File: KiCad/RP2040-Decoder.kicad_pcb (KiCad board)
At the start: 2 copper layers, 25 x 20 mm, 57 parts, among them J1 T0, J10 2, J11 3, J12 4, J13 5, J14 +V, J15 M_OUT_B, J16 M_OUT_A, J17 GND, J18 SWCLK, J19 SWDIO, J2 T1, J20 RUN, J3 0, J4 1, J5 2, J6 3, J7 +3V3, J8 0, J9 1, Q1 T2N7002BK, Q2 T2N7002BK, Q3 T2N7002BK, Q4 T2N7002BK, Q5 T2N7002BK, U1 PJ75AL33SA, U2 BDR6133, U3 W25Q64JVSSIQ, U4 RP2040, Y1 X322512MSB4SI

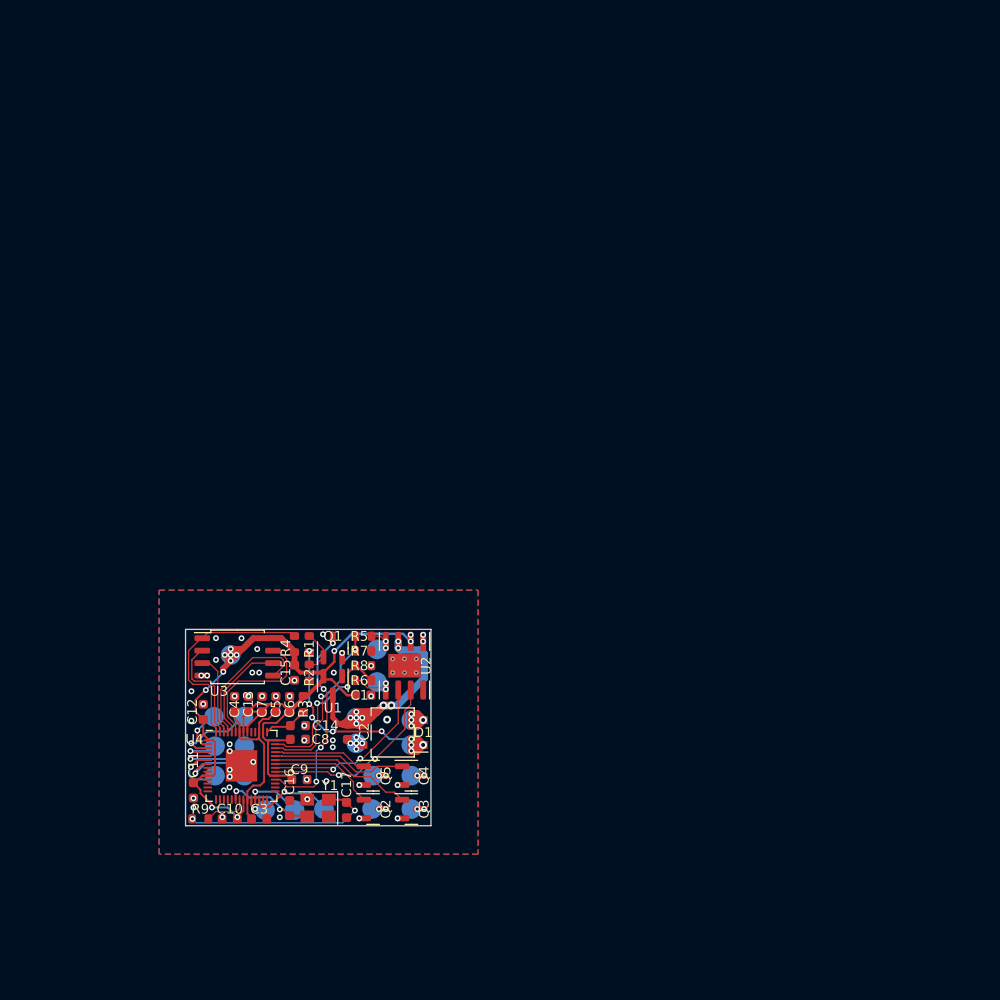
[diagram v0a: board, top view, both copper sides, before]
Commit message: working on PCB
looking to mimic RPi's own minimal PCB
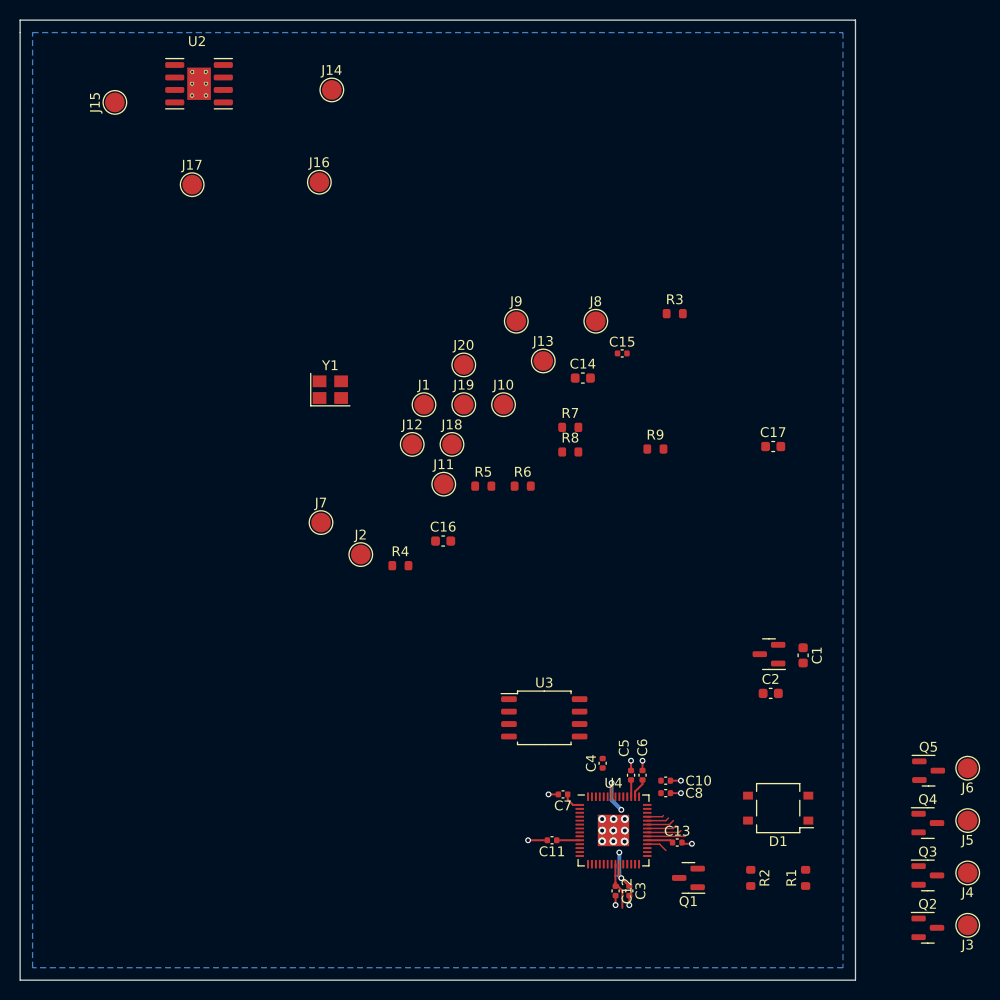
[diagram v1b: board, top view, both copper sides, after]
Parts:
- removed C9: 100n, RP2040-Decoder_Additional_Footprints:C_0603_1608Metric
- C1, C14, C16, C17, C2: footprint RP2040-Decoder_Additional_Footprints:C_0603_1608Metric -> Capacitor_SMD:C_0603_1608Metric
- C10, C11, C12, C13, C15, C3, C4, C7, C8: footprint RP2040-Decoder_Additional_Footprints:C_0603_1608Metric -> Capacitor_SMD:C_0402_1005Metric
- C5, C6: value 10u -> 1u; footprint RP2040-Decoder_Additional_Footprints:C_0603_1608Metric -> Capacitor_SMD:C_0402_1005Metric
- J1, J10, J11, J12, J13, J14, J15, J16, J17, J18, J19, J2, J20, J3, J4, J5, J6, J7, J8, J9: moved to F.Cu
- moved J14 64.0 mm to (152.4, 35.1), turned to 0 degrees
- moved U2 62.9 mm to (138.9, 34.4), turned to 0 degrees
- moved J3 61.8 mm to (217.2, 120.1)
- moved J15 61.8 mm to (130.3, 36.3), turned to 90 degrees
- moved J6 60.6 mm to (217.2, 104.1)
- moved R9 59.7 mm to (185.4, 71.6), turned to 0 degrees
- moved J17 59.3 mm to (138.2, 44.7), turned to 0 degrees
- moved Q2 57.8 mm to (213.1, 120.4)
- moved C17 57.1 mm to (197.4, 71.4), turned to 0 degrees
- moved J4 57.0 mm to (217.2, 114.8)
- moved J5 56.9 mm to (217.2, 109.5)
- moved Q5 56.6 mm to (213.2, 104.4)
- moved J8 56.0 mm to (179.3, 58.6), turned to 0 degrees
- moved R1 55.9 mm to (200.7, 115.3), turned to 90 degrees
- moved R3 54.9 mm to (187.3, 57.8), turned to 0 degrees
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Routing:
- net +3V3: track 92.6 -> 14.1 mm, vias 12 -> 0
- net +V: track 34.5 -> 0.00 mm, vias 9 -> 0
- net Net-(D1-Pad1): track 27.9 -> 0.00 mm, vias 9 -> 0
- net Net-(R4-Pad1): track 22.0 -> 0.00 mm
- net Net-(C17-Pad1): track 20.3 -> 0.00 mm, vias 2 -> 0
- net /GPIO21: track 20.5 -> 2.17 mm, vias 4 -> 0
- net /ADC_EMF_A: track 17.6 -> 0.00 mm, vias 2 -> 0
- net /ADC_EMF_B: track 16.9 -> 0.00 mm, vias 2 -> 0
- net /GPIO22: track 19.5 -> 3.97 mm, vias 2 -> 0
- net Net-(U3-Pad7): track 14.6 -> 0.00 mm
- net Net-(U3-Pad5): track 14.5 -> 0.00 mm
- net /GPIO23: track 17.9 -> 3.51 mm, vias 2 -> 0
- net Net-(D1-Pad2): track 13.1 -> 0.00 mm, vias 4 -> 0
- net /GPIO25: track 14.6 -> 2.84 mm
- net /GPIO26: track 13.8 -> 2.27 mm
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- removed copper zone on F.Cu, net GND
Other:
- board size 25 x 20 mm -> 85.1 x 97.8 mm
- board text removed: "AUX"
- board text removed: "DEBUG"
- board text removed: "GPIO"
- board text removed: "Gabriel Koppenstein RP2040-Decoder"
- board text removed: "M"
- board text removed: "Rev. 0.3"
